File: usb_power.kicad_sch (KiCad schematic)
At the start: 38 parts, among them J1 USB_C_Receptacle_USB2.0_14P, Q1 IRLML6402, SW25 SW_Push_DPDT, U12 CH340N, U13 TP4056-42-ESOP8, U14 SX1308, U15 LM393

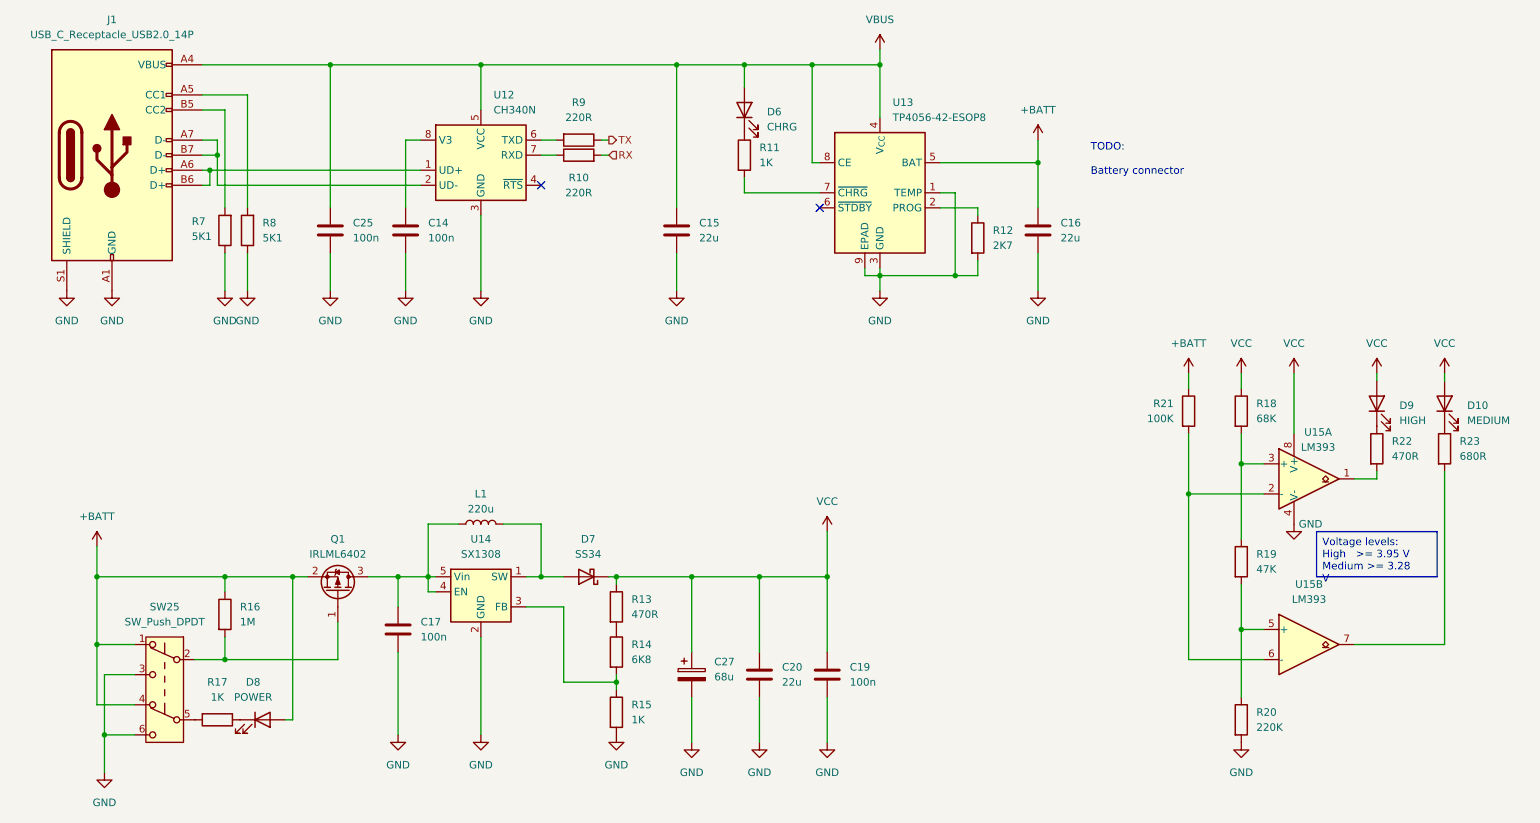
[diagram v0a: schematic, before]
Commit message: HW: Start final placement
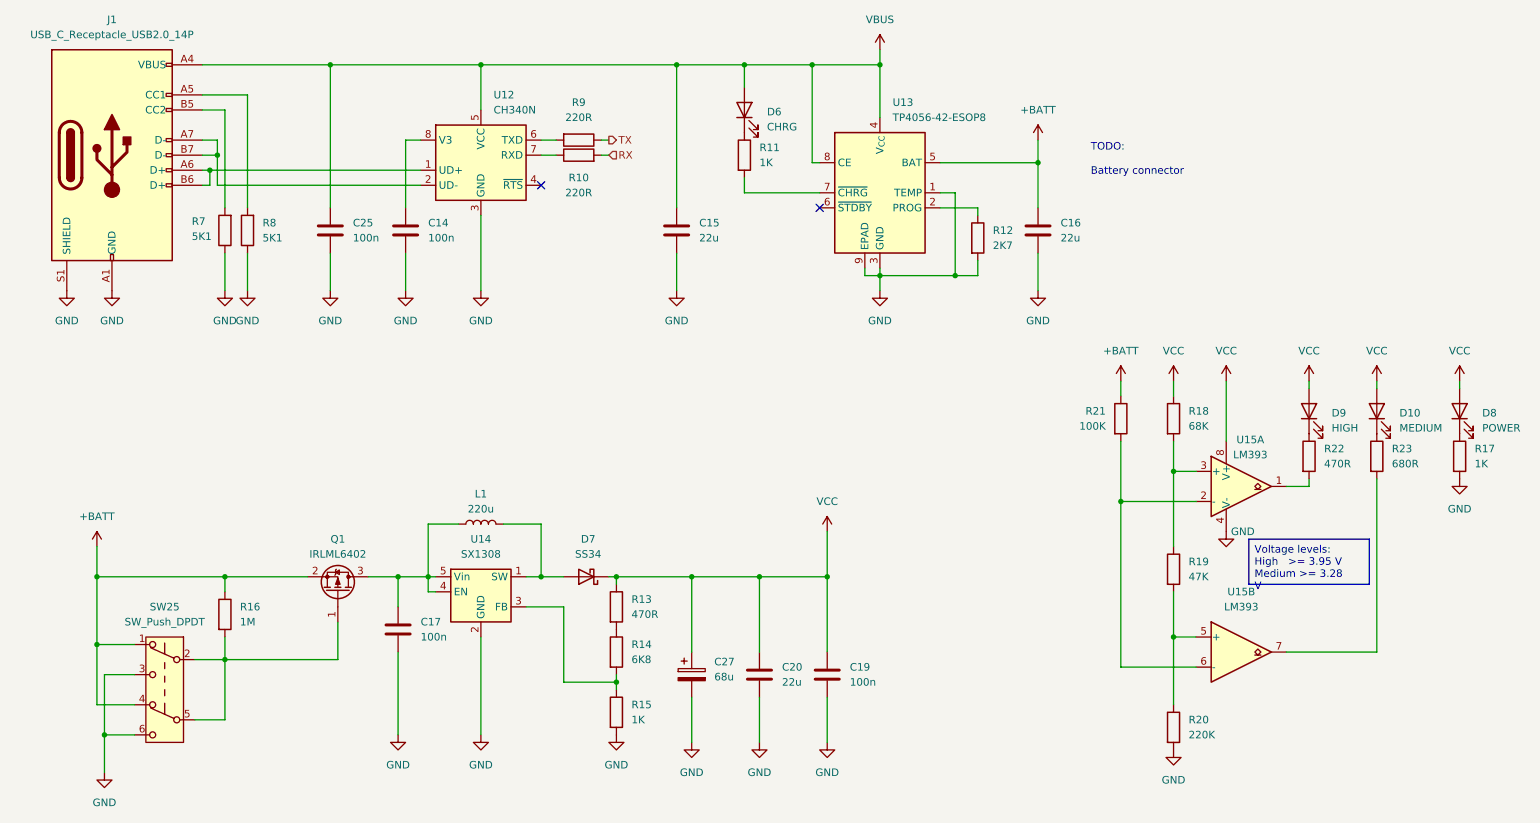
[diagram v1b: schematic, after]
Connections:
- net +BATT: no longer D8.2 (A)
- net GND: now also R17.2
- net VCC: now also D8.2 (A)
- net at SW25.5 (B): now also Q1.1 (G), R16.2, SW25.2 (B); no longer R17.2
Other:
- moved on the sheet: D10, D8, D9, R17, R18, R19, R20, R21, R22, R23, U15A, U15B
